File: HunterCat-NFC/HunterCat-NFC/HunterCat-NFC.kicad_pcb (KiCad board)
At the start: 2 copper layers, 80.7 x 33.5 mm, 71 parts, among them J1 Battery, J2 Conn_01x06_Female, P1 USB_C_Plug_USB2.0, Q1 DMG3415U-7, SW1 RESET, SW2 GPIO, SW3 GPIO1, SW4 GPIO2, U1 ATSAMD21E18A, U2 PN7150B0HN_C11002E-PN7150B0HN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, U3 MCP73831-3-OT, U4 AP2112K-3.3, U5 GD25Q16CEIGR, Y1 27.12Mhz

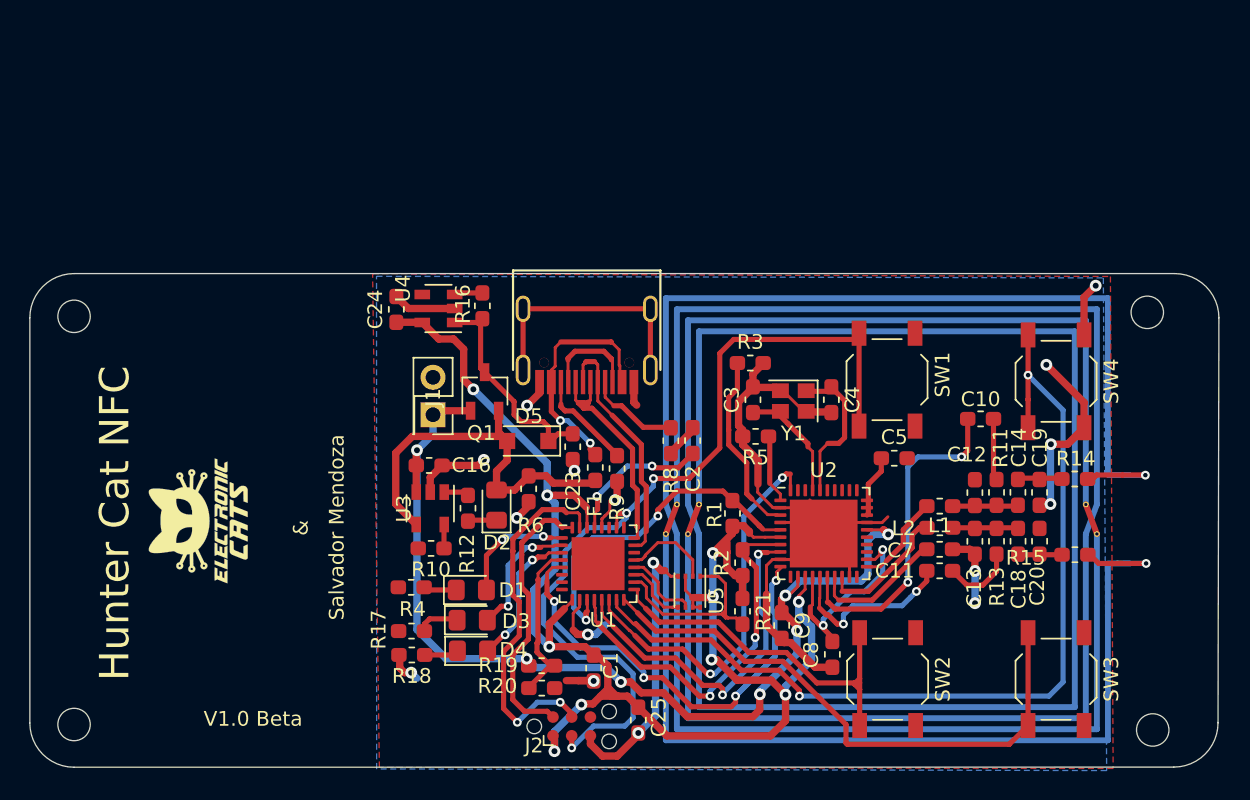
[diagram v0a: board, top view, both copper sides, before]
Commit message: Change Position
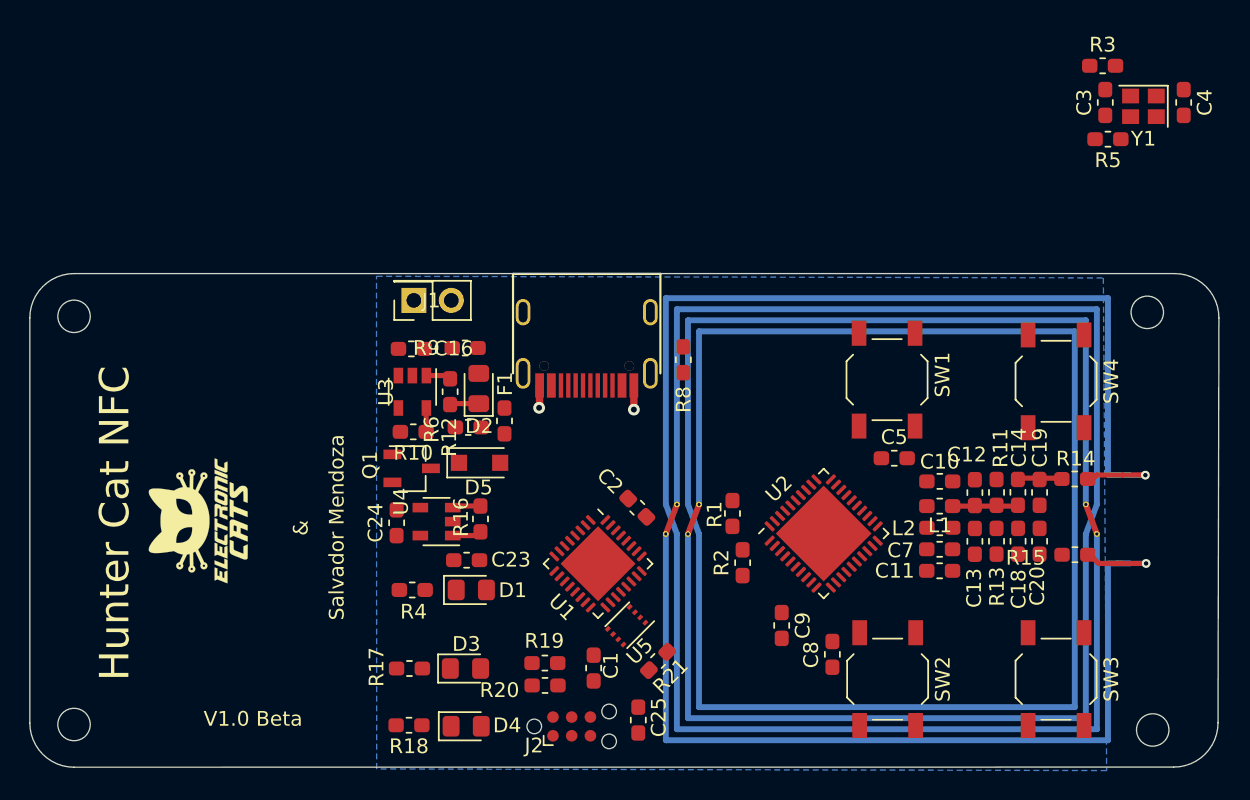
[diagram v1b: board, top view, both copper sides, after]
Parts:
- moved C4 31.3 mm to (158.3, 63.9)
- moved R3 31.3 mm to (152.8, 61.4)
- moved C3 31.3 mm to (153.0, 63.9)
- moved R5 31.3 mm to (153.2, 66.4)
- moved Y1 31.1 mm to (155.6, 64.2)
- moved C24 14.5 mm to (104.9, 92.4)
- moved R16 14.5 mm to (110.6, 92.2)
- moved U4 14.5 mm to (107.6, 92.3)
- moved R9 13.2 mm to (109.5, 80.5), turned to 0 degrees
- moved C23 10.5 mm to (109.6, 95.0), turned to 0 degrees
- moved R10 8.00 mm to (106.0, 86.2)
- moved U3 8.00 mm to (106.0, 83.5)
- moved D2 8.00 mm to (110.5, 83.3)
- moved R12 8.00 mm to (108.5, 83.5)
- moved C16 8.00 mm to (105.9, 80.6)
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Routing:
- net GND: track 123.6 -> 3.16 mm, vias 16 -> 2
- net +3V3: track 107.3 -> 0.00 mm, vias 10 -> 0
- net +BATT: track 69.9 -> 0.00 mm, vias 7 -> 0
- net /GPIO2: track 62.0 -> 0.00 mm, vias 2 -> 0
- net /RST: track 60.0 -> 0.00 mm, vias 3 -> 0
- net /GPIO1: track 39.1 -> 0.00 mm
- net /VEN: track 36.2 -> 0.00 mm, vias 4 -> 0
- net /CLK: track 26.9 -> 0.00 mm, vias 2 -> 0
- net VBUS: track 26.9 -> 0.00 mm
- net /SCL: track 25.8 -> 0.00 mm, vias 2 -> 0
- net /GPIO: track 25.7 -> 0.00 mm
- net /SWCLK: track 24.7 -> 0.00 mm, vias 2 -> 0
- net /IRQ: track 24.5 -> 0.00 mm, vias 2 -> 0
- net /SDA: track 23.4 -> 0.00 mm, vias 2 -> 0
- net /RXP: track 23.0 -> 0.00 mm, vias 2 -> 0
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- added copper zone on In1.Cu, net GND
- removed copper zone on F.Cu, net GND
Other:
- copper layers 2 -> 4
